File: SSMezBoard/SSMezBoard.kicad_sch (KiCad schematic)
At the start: 2 parts, among them U1 DFRobot_DC_Controller

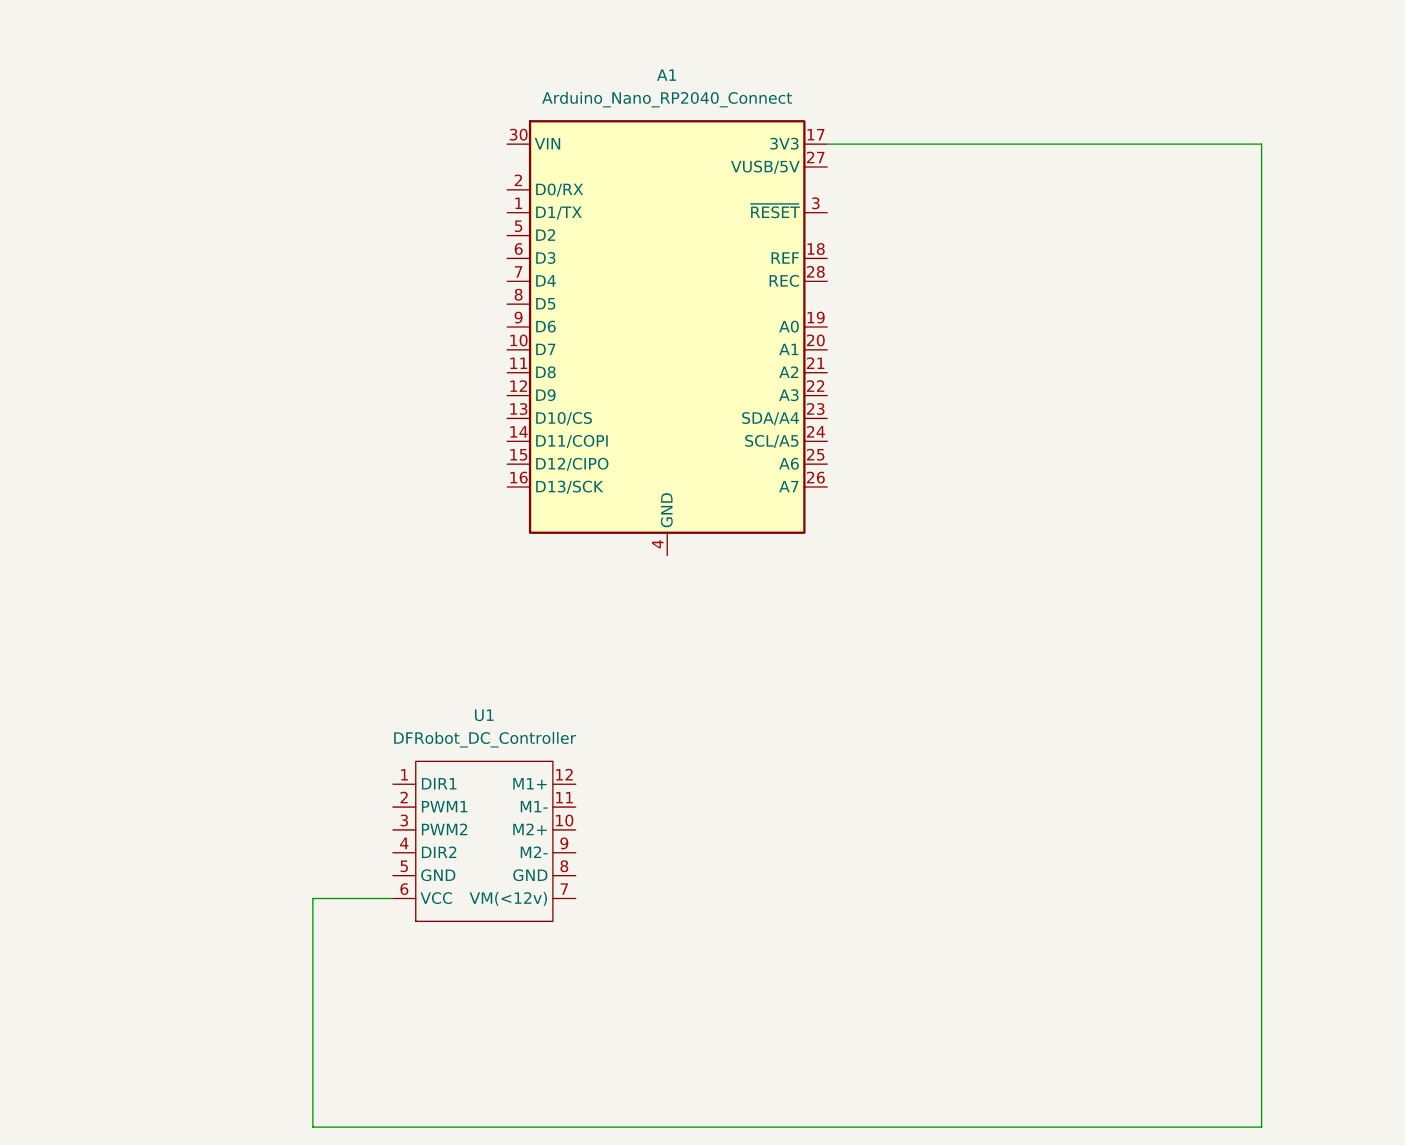
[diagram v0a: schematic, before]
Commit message: Sort of ready for JLCPCB
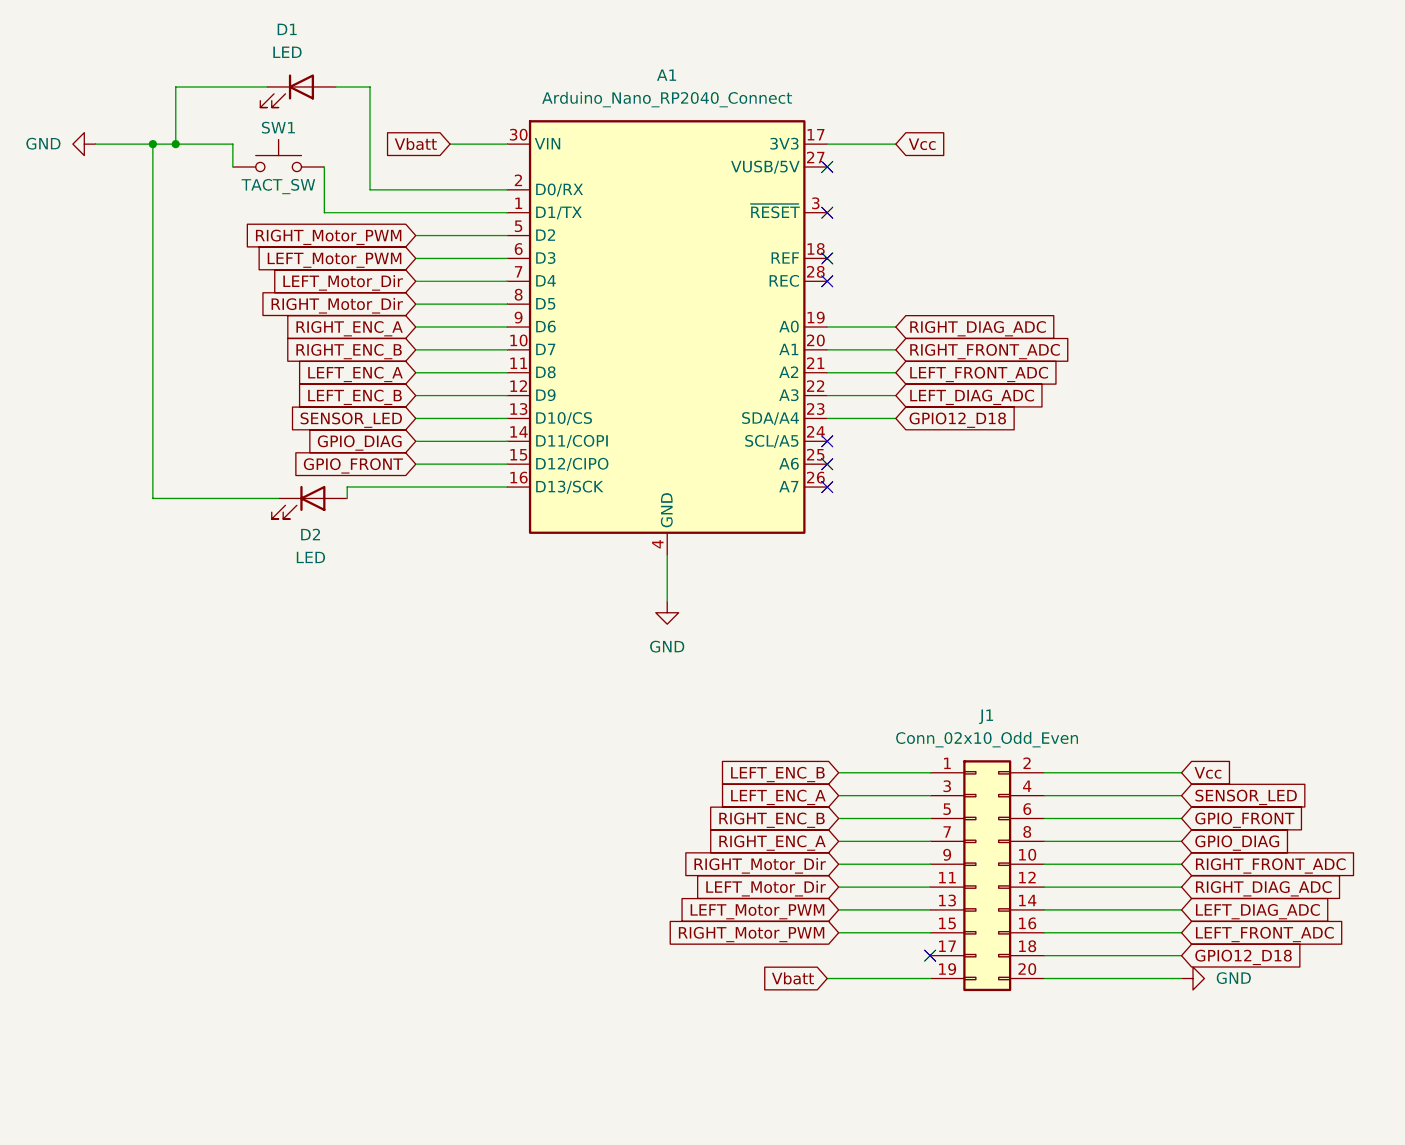
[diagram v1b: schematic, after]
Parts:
- removed U1: DFRobot_DC_Controller, PBFootPrintLibrary:DFRobot_DC_Controller, symbol PB_Library:DFRobot_DC_Motor_Controller
- added D1, D2: LED, LED_THT:LED_D5.0mm, symbol Device:LED
- added J1: Conn_02x10_Odd_Even, Connector_PinHeader_2.54mm:PinHeader_2x10_P2.54mm_Horizontal, symbol Connector_Generic:Conn_02x10_Odd_Even
- added SW1: TACT_SW, Button_Switch_THT:SW_PUSH_6mm, symbol PB_Library:Tact_Switch_6mm
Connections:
- net at A1.1 (D1/TX): now also SW1.2 (B)
- net RIGHT_ENC_B: now reaches A1.10 (D7)
- net RIGHT_ENC_B: now also J1.5 (Pin_5)
- net LEFT_ENC_A: now reaches A1.11 (D8)
- net LEFT_ENC_A: now also J1.3 (Pin_3)
- net LEFT_ENC_B: now reaches A1.12 (D9)
- net LEFT_ENC_B: now also J1.1 (Pin_1)
- net SENSOR_LED: now reaches A1.13 (D10/CS)
- net SENSOR_LED: now also J1.4 (Pin_4)
- net GPIO_DIAG: now reaches A1.14 (D11/COPI)
- net GPIO_DIAG: now also J1.8 (Pin_8)
- net GPIO_FRONT: now reaches A1.15 (D12/CIPO)
- net GPIO_FRONT: now also J1.6 (Pin_6)
- net at A1.16 (D13/SCK): now also D2.2 (A)
- net Vcc: now reaches A1.17 (3V3)
- net Vcc: now also J1.2 (Pin_2)
- net RIGHT_DIAG_ADC: now reaches A1.19 (A0)
- net RIGHT_DIAG_ADC: now also J1.12 (Pin_12)
- net at A1.2 (D0/RX): now also D1.2 (A)
- net RIGHT_FRONT_ADC: now reaches A1.20 (A1)
- net RIGHT_FRONT_ADC: now also J1.10 (Pin_10)
- net LEFT_FRONT_ADC: now reaches A1.21 (A2)
- net LEFT_FRONT_ADC: now also J1.16 (Pin_16)
- net LEFT_DIAG_ADC: now reaches A1.22 (A3)
- net LEFT_DIAG_ADC: now also J1.14 (Pin_14)
- net GPIO12_D18: now reaches A1.23 (SDA/A4)
- net GPIO12_D18: now also J1.18 (Pin_18)
- net GND: now reaches A1.29 (GND), A1.4 (GND)
- net GND: now also D1.1 (K), D2.1 (K), J1.20 (Pin_20), SW1.1 (A)
- net Vbatt: now reaches A1.30 (VIN)
- net Vbatt: now also J1.19 (Pin_19)
- net RIGHT_Motor_PWM: now reaches A1.5 (D2)
- net RIGHT_Motor_PWM: now also J1.15 (Pin_15)
- net LEFT_Motor_PWM: now reaches A1.6 (D3)
- net LEFT_Motor_PWM: now also J1.13 (Pin_13)
- net LEFT_Motor_Dir: now reaches A1.7 (D4)
- net LEFT_Motor_Dir: now also J1.11 (Pin_11)
- net RIGHT_Motor_Dir: now reaches A1.8 (D5)
- net RIGHT_Motor_Dir: now also J1.9 (Pin_9)
- net RIGHT_ENC_A: now reaches A1.9 (D6)
- net RIGHT_ENC_A: now also J1.7 (Pin_7)
- no-connect marks 0 -> 8
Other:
- title: (none) -> Carrier Board for the Ardunio Nano RP2040 Connect
